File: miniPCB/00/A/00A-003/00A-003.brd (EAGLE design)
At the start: 13 parts

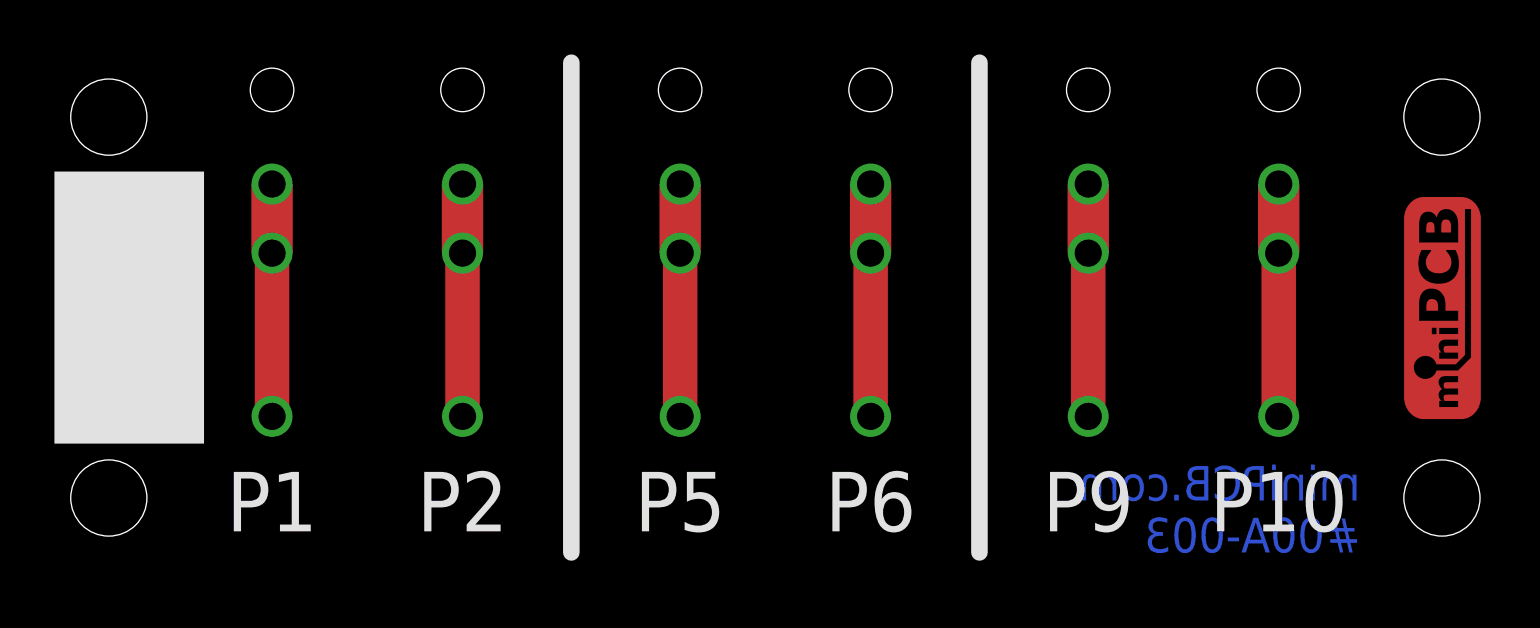
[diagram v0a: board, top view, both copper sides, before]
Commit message: NM.28JAN2023
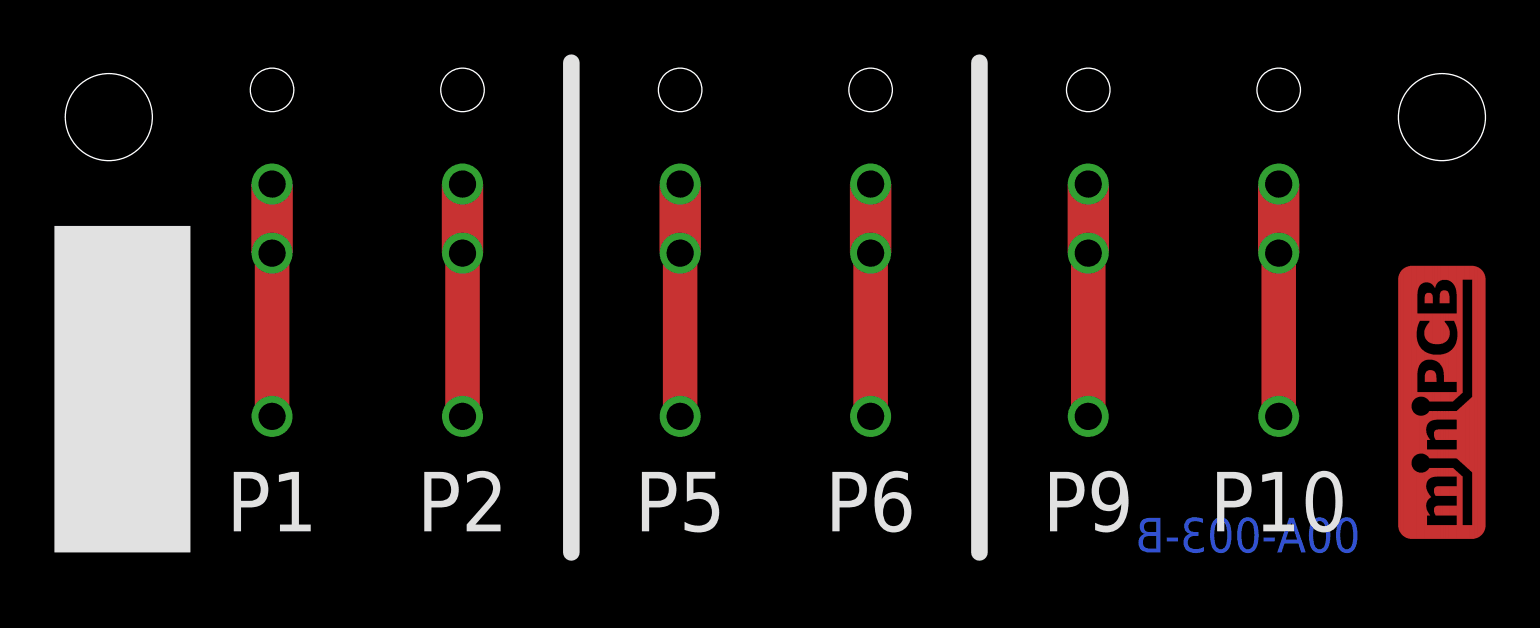
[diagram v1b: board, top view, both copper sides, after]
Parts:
- removed U$1: MINIPCB_LOGO, nolan-utsa:MINIPCB_LOGO
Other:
- board text added: "00A-003-B"
- board text removed: "miniPCB.com #00A-003"
